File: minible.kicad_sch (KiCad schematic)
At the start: 31 parts, among them U2 nRF52833_QDxx, Y2 Crystal_GND24

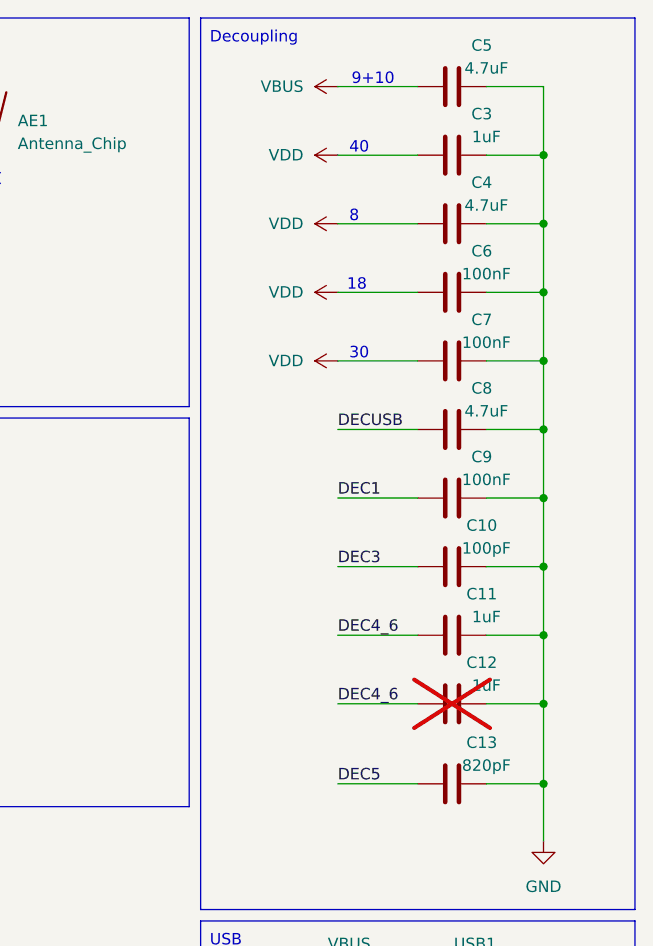
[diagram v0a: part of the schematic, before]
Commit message: finish pcb
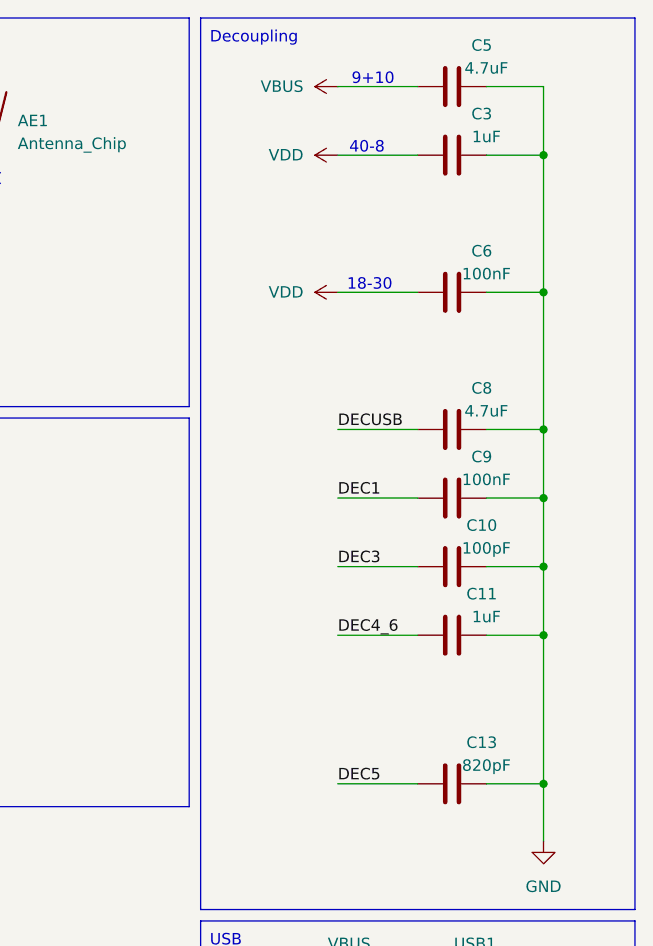
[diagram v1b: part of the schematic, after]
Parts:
- removed C12: 1uF, Capacitor_SMD:C_0603_1608Metric, symbol Device:C
- removed C4: 4.7uF, Capacitor_SMD:C_0603_1608Metric, symbol Device:C
- removed C7: 100nF, Capacitor_SMD:C_0603_1608Metric, symbol Device:C
- C10: footprint Capacitor_SMD:C_0402_1005Metric -> Capacitor_SMD:C_0201_0603Metric; Supplier Part C106200 -> C272870
- C11, C3: footprint Capacitor_SMD:C_0603_1608Metric -> Capacitor_SMD:C_0201_0603Metric; Supplier Part C29936 -> C76930
- C13: footprint Capacitor_SMD:C_0402_1005Metric -> Capacitor_SMD:C_0201_0603Metric; Supplier Part C3899834 -> C2836759
- C14: footprint Capacitor_SMD:C_0402_1005Metric -> Capacitor_SMD:C_0201_0603Metric; Supplier Part C1550 -> C20069198
- C15: footprint Capacitor_SMD:C_0402_1005Metric -> Capacitor_SMD:C_0201_0603Metric; Supplier Part C880658 -> C48642883
- C16, C17: footprint Capacitor_SMD:C_0402_1005Metric -> Capacitor_SMD:C_0201_0603Metric; Supplier Part C696888 -> C50391
- C5, C8: footprint Capacitor_SMD:C_0603_1608Metric -> Capacitor_SMD:C_0402_1005Metric; Supplier Part C19666 -> C318563
- C6, C9: footprint Capacitor_SMD:C_0603_1608Metric -> Capacitor_SMD:C_0201_0603Metric; Supplier Part C14663 -> C307380
- L1: footprint Inductor_SMD:L_0402_1005Metric -> Inductor_SMD:L_0201_0603Metric; Supplier Part C7427063 -> C3910459
- L2: footprint Inductor_SMD:L_0402_1005Metric -> Inductor_SMD:L_0201_0603Metric; Supplier Part C436294 -> C52109740
- R1, R2: footprint Resistor_SMD:R_0603_1608Metric -> Resistor_SMD:R_0201_0603Metric; Supplier Part C2907044 -> C473460
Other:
- note added: "18-30"
- note added: "40-8"
- note removed: "18"
- note removed: "30"
- note removed: "40"
- note removed: "8"
